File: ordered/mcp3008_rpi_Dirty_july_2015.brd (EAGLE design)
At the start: 49.8 x 22.2 mm, 10 parts

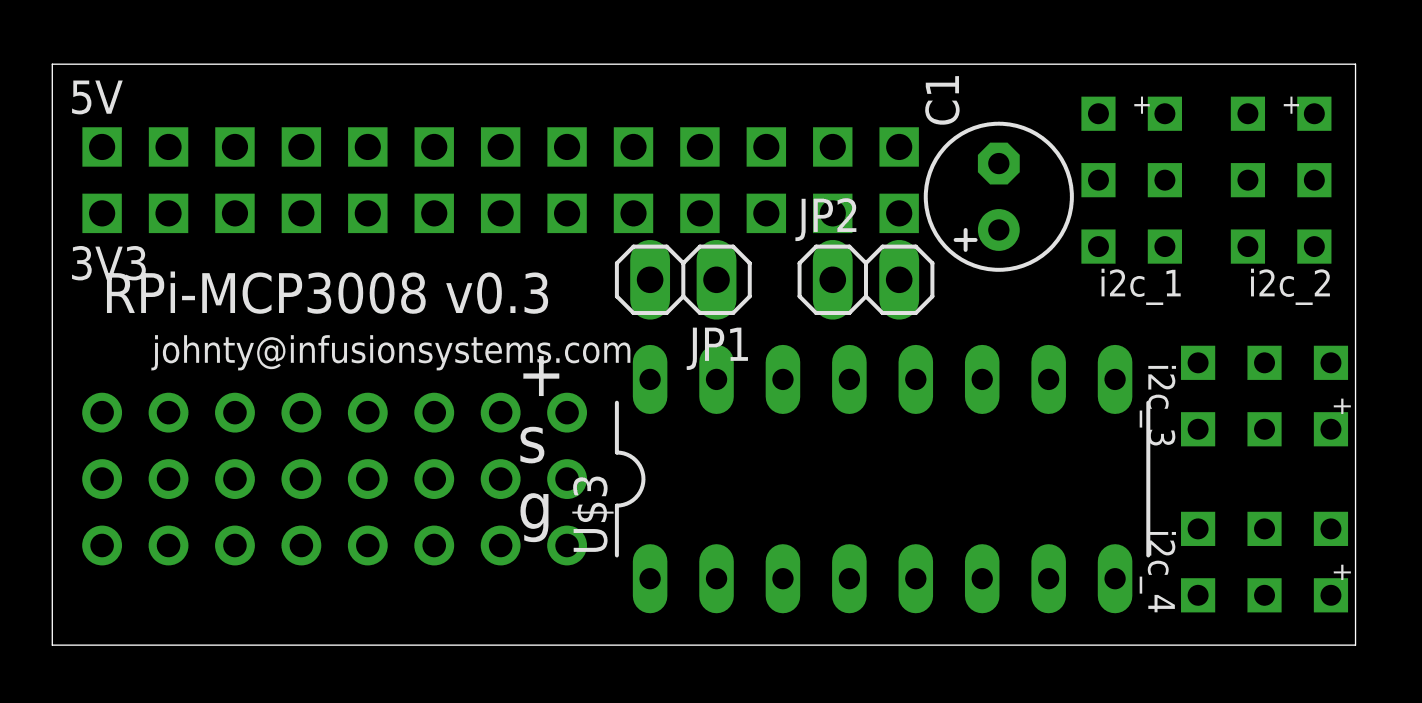
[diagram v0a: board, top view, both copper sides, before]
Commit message: i2c board complete
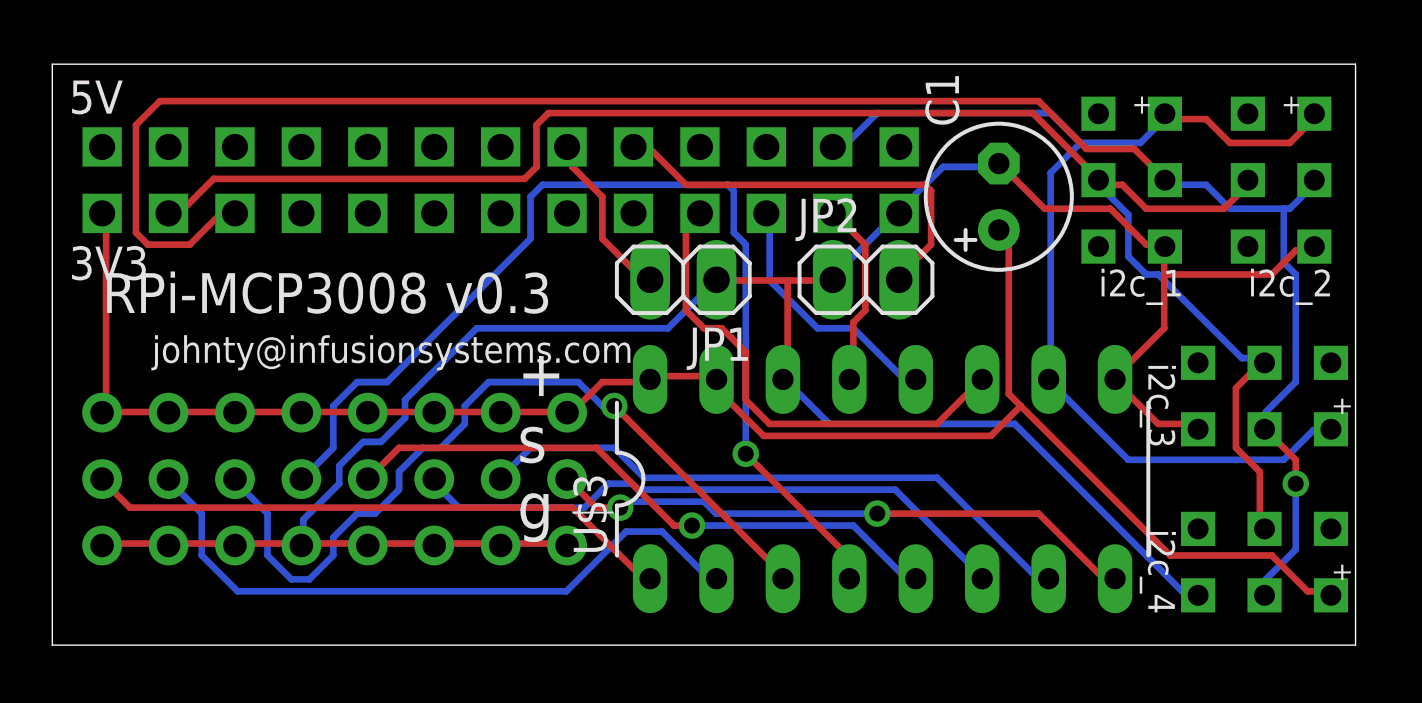
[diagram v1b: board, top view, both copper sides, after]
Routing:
- net GND: track 0.00 -> 99.3 mm
- net N$14: track 0.00 -> 72.7 mm, vias 0 -> 1
- net VCC: track 0.00 -> 67.3 mm
- net N$15: track 0.00 -> 63.6 mm
- net N$12: track 0.00 -> 43.1 mm
- net N$4: track 0.00 -> 39.8 mm, vias 0 -> 1
- net N$3: track 0.00 -> 31.0 mm, vias 0 -> 1
- net N$2: track 0.00 -> 25.5 mm
- net N$7: track 0.00 -> 23.6 mm
- net N$5: track 0.00 -> 23.6 mm, vias 0 -> 1
- net N$6: track 0.00 -> 23.4 mm
- net N$8: track 0.00 -> 22.7 mm, vias 0 -> 2
- net N$1: track 0.00 -> 22.7 mm
- net N$11: track 0.00 -> 18.8 mm
- net N$16: track 0.00 -> 15.9 mm
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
